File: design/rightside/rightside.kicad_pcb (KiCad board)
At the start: 4 copper layers, 142.6 x 96.2 mm, 227 parts, among them IC2 XC9148G50CER-G, IC3 nRF52833-QDAA-R7, IC4 74AHCT125PW,118, IC5 MCP23018T-E_SS, IC6 XC9291B33D1R-G, J1 USB_C_Receptacle_USB2.0_16P, J2 Battery Pos, J3 Battery Neg, J4 OLED_128x32, J6 Conn_01x04, J7 F32Q-1A7H1-11012, U1 BQ27441-G1, U2 BQ24072RGT, U3 USB6B1, U5 PEC11L-4015F-S0015, U6 PEC11L-4015F-S0015, Y1 ECS-320-8-37B2-JTY-TR

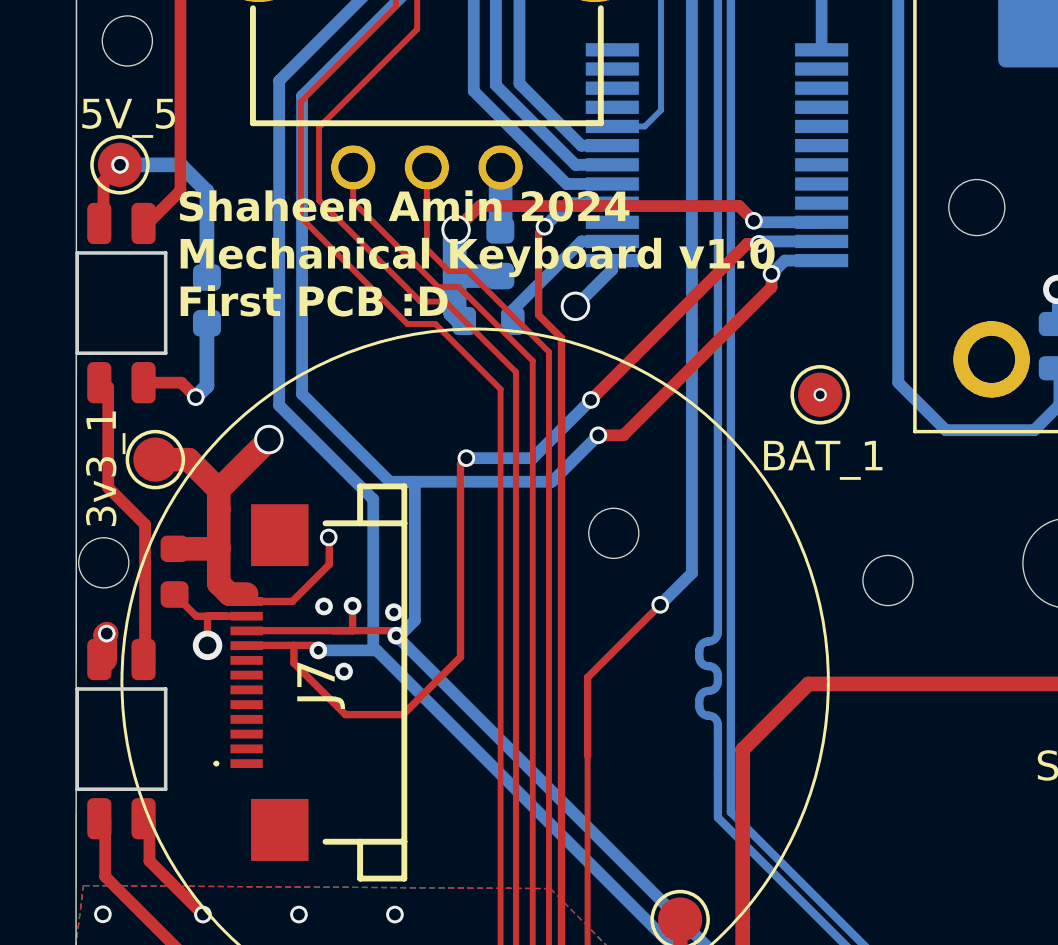
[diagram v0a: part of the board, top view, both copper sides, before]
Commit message: LS RS no error
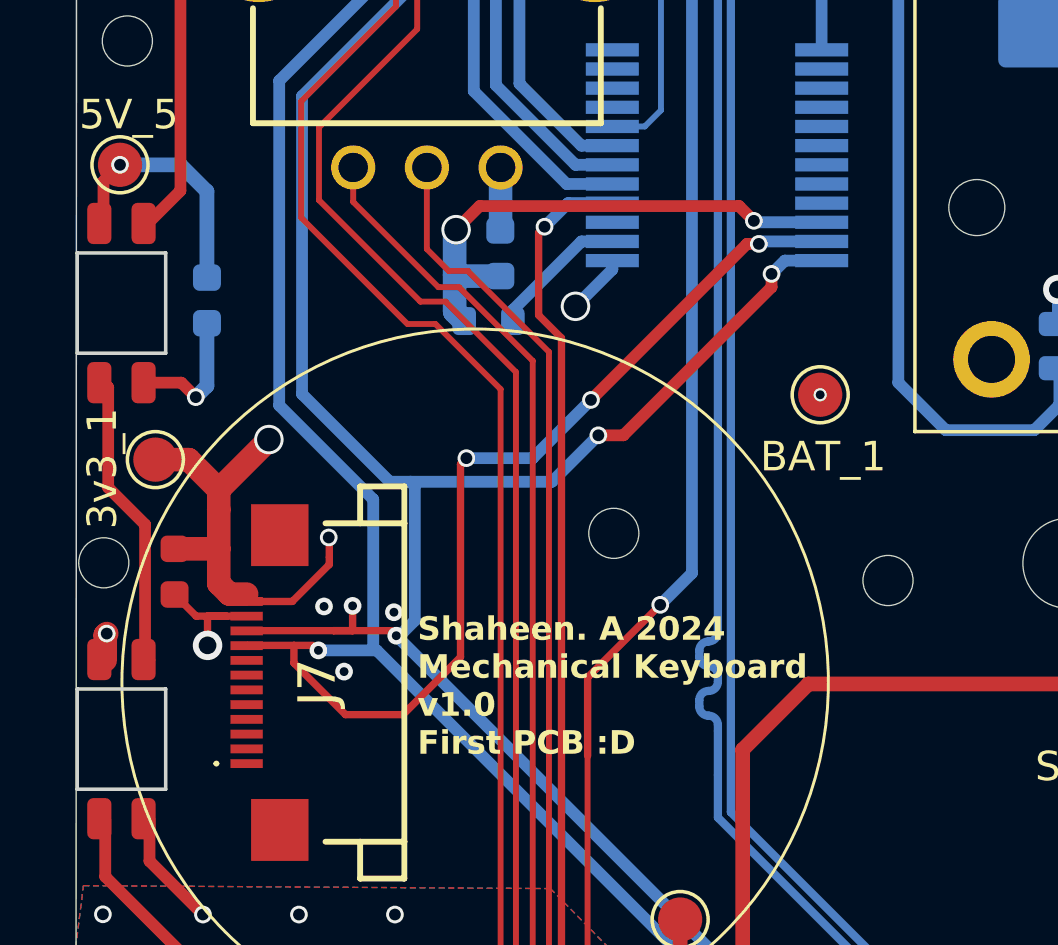
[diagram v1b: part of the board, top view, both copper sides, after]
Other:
- board text added: "Shaheen. A 2024 Mechanical Keyboard v1.0 First PCB :D"
- board text removed: "Shaheen Amin 2024 Mechanical Keyboard v1.0 First PCB :D"
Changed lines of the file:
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@@
 		(layer "Edge.Cuts")
 	)
-	(gr_text "Shaheen Amin 2024\nMechanical Keyboard v1.0\nFirst PCB :D"
-		(at 242.440969 130.830719 0)
+	(gr_text "Shaheen. A 2024\nMechanical Keyboard\nv1.0\nFirst PCB :D"
+		(at 250.6005 145.653652 0)
 		(layer "F.SilkS")
 		(effects
 			(font
-				(size 1 1)
-				(thickness 0.25)
+				(size 0.8 0.8)
+				(thickness 0.2)
 				(bold yes)
 			)
@@
 		(polygon
 			(pts
-				(xy 248.218225 172.09476) (xy 248.228225 173.19476) (xy 251.758225 173.23476) (xy 251.788225 170.28476)
-				(xy 251.670969 167.920719) (xy 251.720969 167.180719) (xy 255.100969 167.170719) (xy 257.070969 166.960719)
-				(xy 258.878225 165.60476) (xy 258.678225 164.93476) (xy 255.310969 164.200719) (xy 251.970969 163.870719)
-				(xy 251.530969 165.450719) (xy 250.000969 166.110719) (xy 250.098225 168.29476) (xy 250.260969 171.980719)
+				(xy 248.221636 172.469948) (xy 248.228225 173.19476) (xy 251.758225 173.23476) (xy 251.788225 170.28476)
+				(xy 251.901793 168.151543) (xy 252.8505 167.180719) (xy 254.3505 167.170719) (xy 255.725781 165.615531)
+				(xy 258.878225 165.60476) (xy 258.678225 164.93476) (xy 255.1505 164.336783) (xy 254.480437 165.545781)
+				(xy 252.0005 165.746349) (xy 251.845029 166.583418) (xy 250.098225 168.29476) (xy 250.277503 172.355175)
 			)
 		)
